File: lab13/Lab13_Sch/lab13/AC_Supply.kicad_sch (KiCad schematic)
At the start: 10 parts, among them U4 4N35

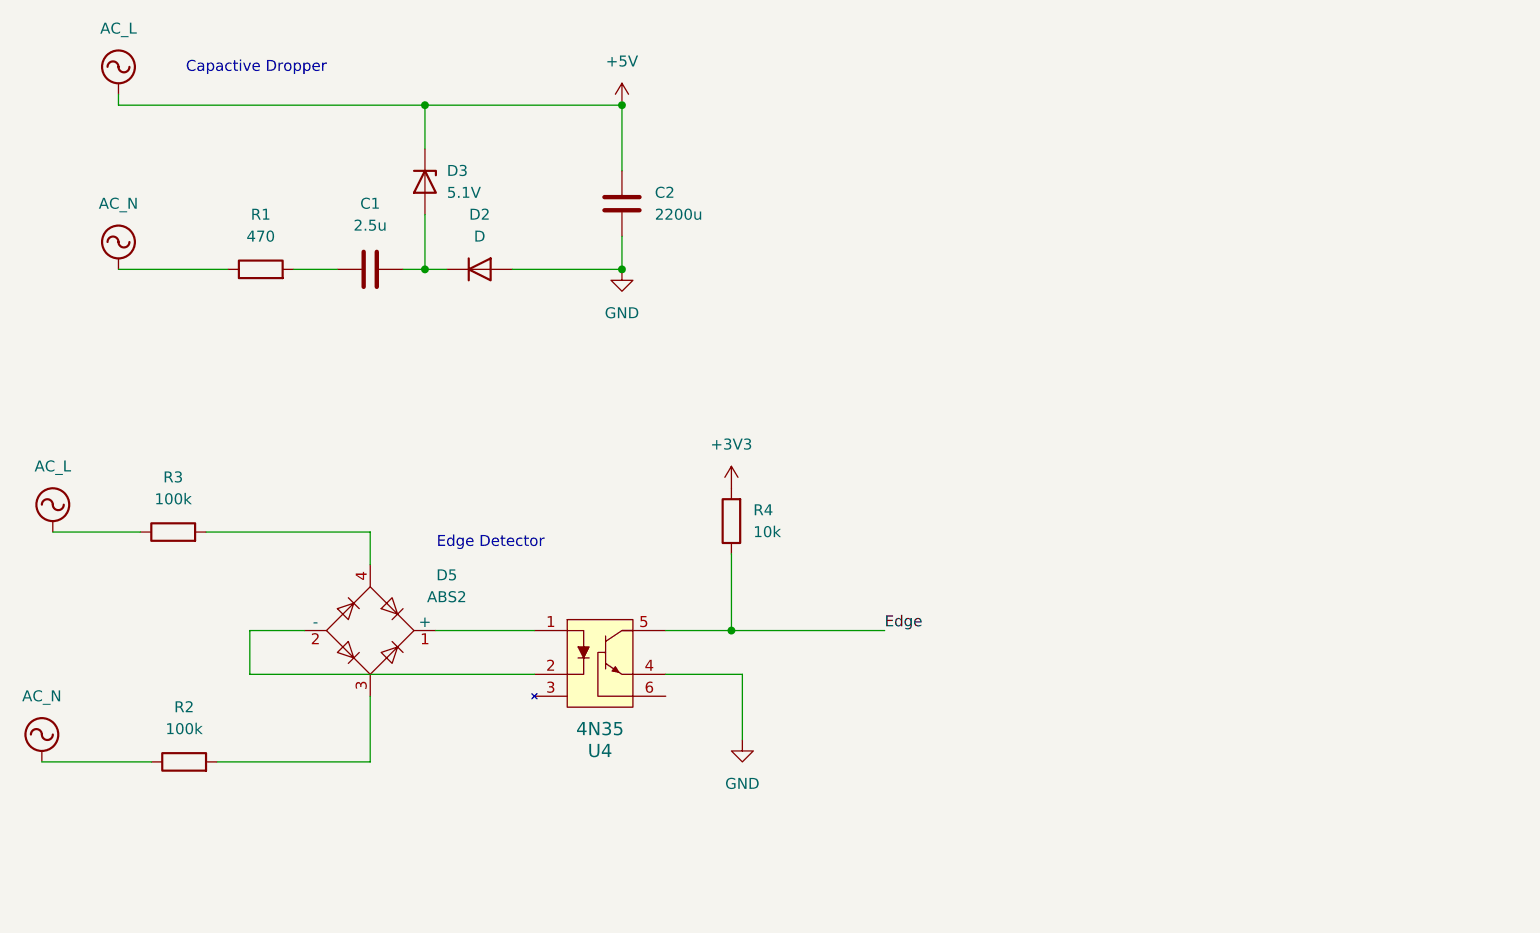
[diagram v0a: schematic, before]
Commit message: Finish lab13 start lab 14
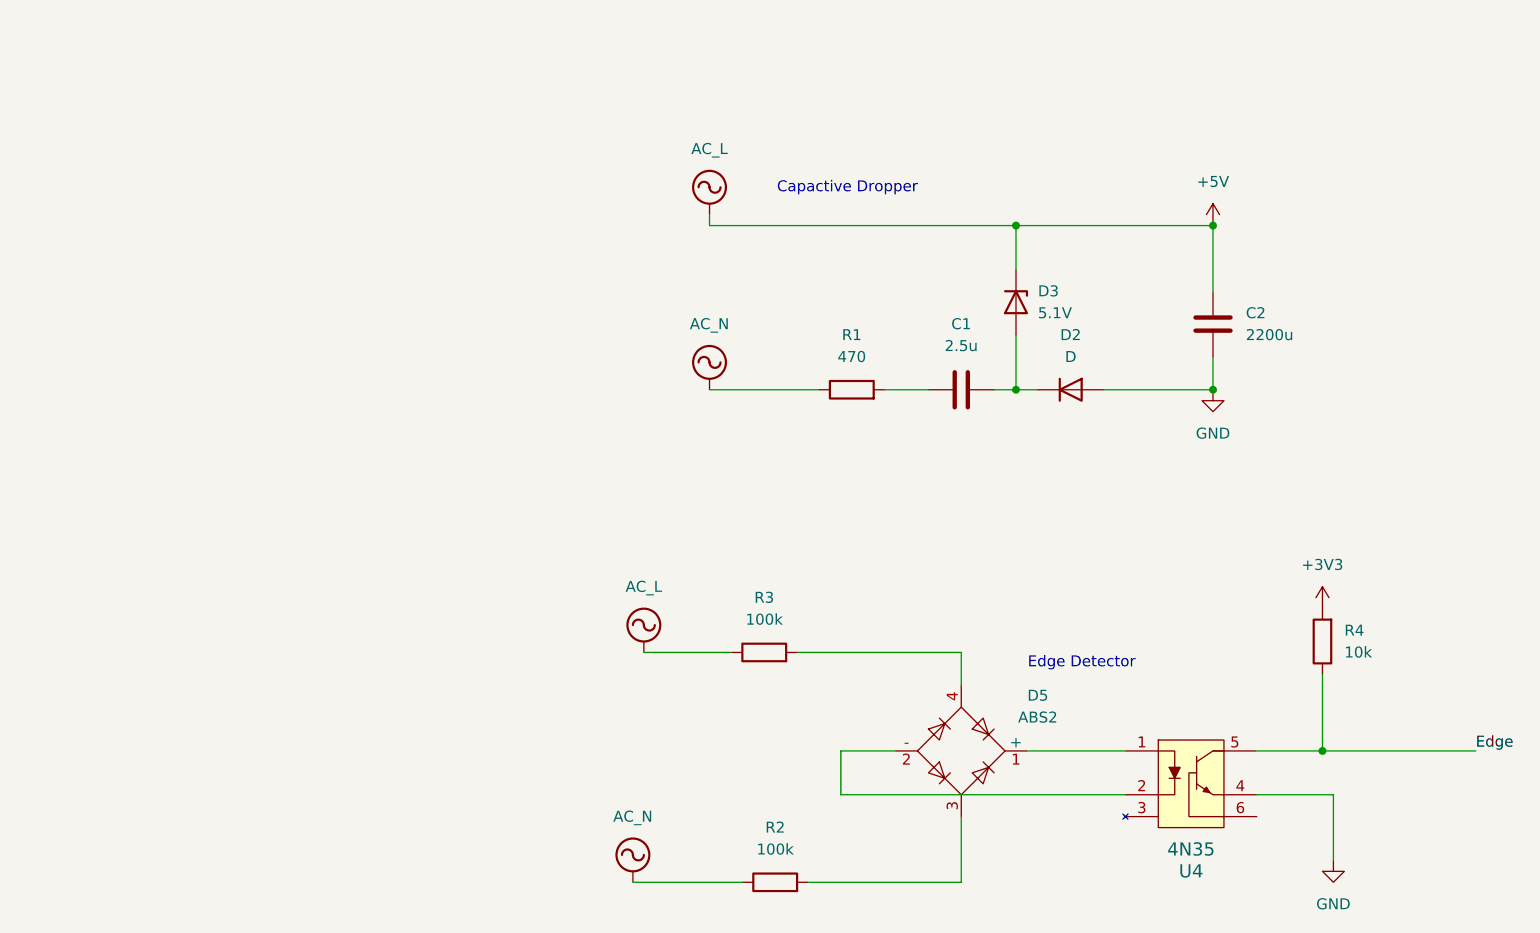
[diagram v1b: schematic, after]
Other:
- company: (none) -> CWRU
- title: (none) -> Lab 13: Digital Heating Pad Control
- moved on the sheet: C1, C2, D2, D3, D5, R1, R2, R3, R4, U4
